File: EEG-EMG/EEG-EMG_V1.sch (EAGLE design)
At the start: 61 parts, among them IC1 MCP6V31, IC11 LM7332MA, IC2 MCP6V31, IC3 MCP6V31, IC4 MCP6V31, IC6 MCP3912, Q7 CSM-3X-CRYSTALCSM-3X, U2 BGM111-VISUAL-A

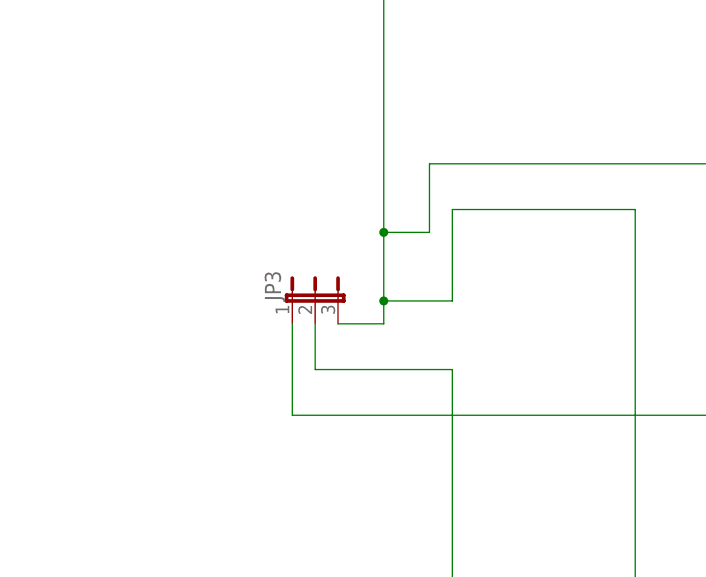
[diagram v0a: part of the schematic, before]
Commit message: Completed Board - Basic Functionality V1
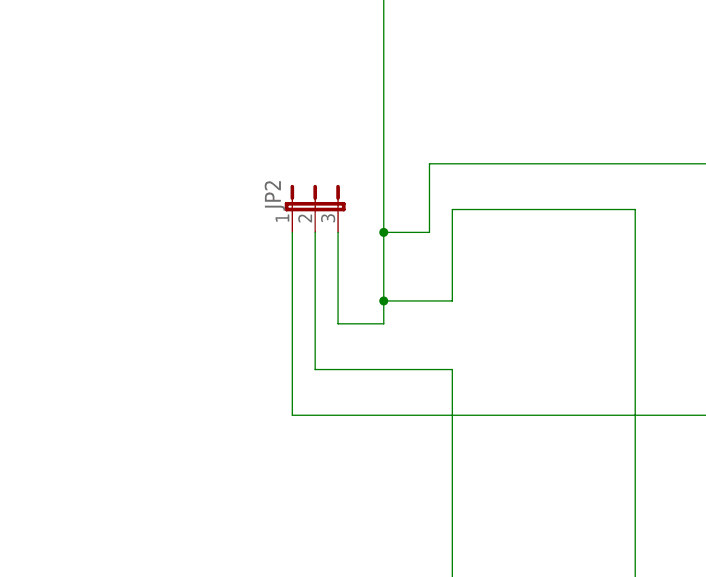
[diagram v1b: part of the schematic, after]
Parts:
- removed JP3: (no value), jumper:JP2E
- added JP2: (no value), jumper:JP2W
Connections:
- net EMG1+: now also JP2.1; no longer JP3.1
- net EMG2+: now also JP2.2; no longer JP3.2
- net REF: now also JP2.3; no longer JP3.3
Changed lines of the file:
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@@
 <part name="GND29" library="SparkFun-Aesthetics" deviceset="GND" device=""/>
 <part name="J2" library="tag-connect" deviceset="TC2030" device="-MCP-NL"/>
-<part name="JP3" library="jumper" deviceset="JP2E" device=""/>
 <part name="BAT2" library="SMTU-2032-1" deviceset="2032" device=""/>
+<part name="JP2" library="jumper" deviceset="JP2W" device=""/>
 </parts>
 <sheets>
@@
 <instance part="GND29" gate="1" x="1013.46" y="-233.68"/>
 <instance part="J2" gate="G$1" x="982.98" y="-228.6" rot="R180"/>
-<instance part="JP3" gate="1" x="383.54" y="-299.72"/>
 <instance part="BAT2" gate="G$1" x="381" y="-43.18" rot="R180"/>
+<instance part="JP2" gate="1" x="383.54" y="-289.56"/>
 </instances>
 <busses>
@@
 <wire x1="472.44" y1="-299.72" x2="472.44" y2="-312.42" width="0.1524" layer="91"/>
 <wire x1="472.44" y1="-312.42" x2="381" y2="-312.42" width="0.1524" layer="91"/>
-<pinref part="JP3" gate="1" pin="1"/>
-<wire x1="381" y1="-302.26" x2="381" y2="-312.42" width="0.1524" layer="91"/>
+<pinref part="JP2" gate="1" pin="1"/>
+<wire x1="381" y1="-292.1" x2="381" y2="-312.42" width="0.1524" layer="91"/>
 </segment>
 </net>
@@
 <wire x1="398.78" y1="-307.34" x2="398.78" y2="-429.26" width="0.1524" layer="91"/>
 <wire x1="398.78" y1="-429.26" x2="497.84" y2="-429.26" width="0.1524" layer="91"/>
-<pinref part="JP3" gate="1" pin="2"/>
 <wire x1="398.78" y1="-307.34" x2="383.54" y2="-307.34" width="0.1524" layer="91"/>
-<wire x1="383.54" y1="-307.34" x2="383.54" y2="-302.26" width="0.1524" layer="91"/>
+<pinref part="JP2" gate="1" pin="2"/>
+<wire x1="383.54" y1="-292.1" x2="383.54" y2="-307.34" width="0.1524" layer="91"/>
 </segment>
 </net>
@@
 <wire x1="391.16" y1="-177.8" x2="391.16" y2="-292.1" width="0.1524" layer="91"/>
 <junction x="439.42" y="-177.8"/>
-<pinref part="JP3" gate="1" pin="3"/>
 <wire x1="391.16" y1="-292.1" x2="391.16" y2="-299.72" width="0.1524" layer="91"/>
 <wire x1="391.16" y1="-299.72" x2="391.16" y2="-302.26" width="0.1524" layer="91"/>
@@
 <wire x1="398.78" y1="-299.72" x2="391.16" y2="-299.72" width="0.1524" layer="91"/>
 <junction x="391.16" y="-299.72"/>
-</segment>
-</net>
+<pinref part="JP2" gate="1" pin="3"/>
+<wire x1="386.08" y1="-292.1" x2="386.08" y2="-302.26" width="0.1524" layer="91"/>
+</segment>
+</net>
